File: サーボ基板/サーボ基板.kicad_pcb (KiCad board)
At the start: 2 copper layers, 120 x 170.1 mm, 83 parts, among them J1 Conn_01x02, J10 Conn_02x10, J11 Conn_01x03_Pin, J12 Conn_01x03_Pin, J13 Conn_01x03_Pin, J14 Conn_01x03_Pin, J15 Conn_01x03_Pin, J16 Conn_01x03_Pin, J17 Conn_01x05, J18 Conn_01x05, J19 Conn_01x04, J2 Conn_01x03, J20 Conn_01x04, J21 Conn_01x04, J3 Conn_01x03, J4 Conn_01x03, J5 Conn_01x03, J6 Conn_01x05_Pin, J9 Conn_01x03, SW1 SW_Push, SW2 SW_Push, SW3 SW_Push, SW4 SW_Push, U1 SeeeduinoXIAO RP2040, U10 SN74HC241DW, U2 DEV-16771, U3 SeeeduinoXIAO RP2040, U4 AD8226ARZ, U5 AD8226ARZ, U8 ADuM121N, U9 ADuM121N

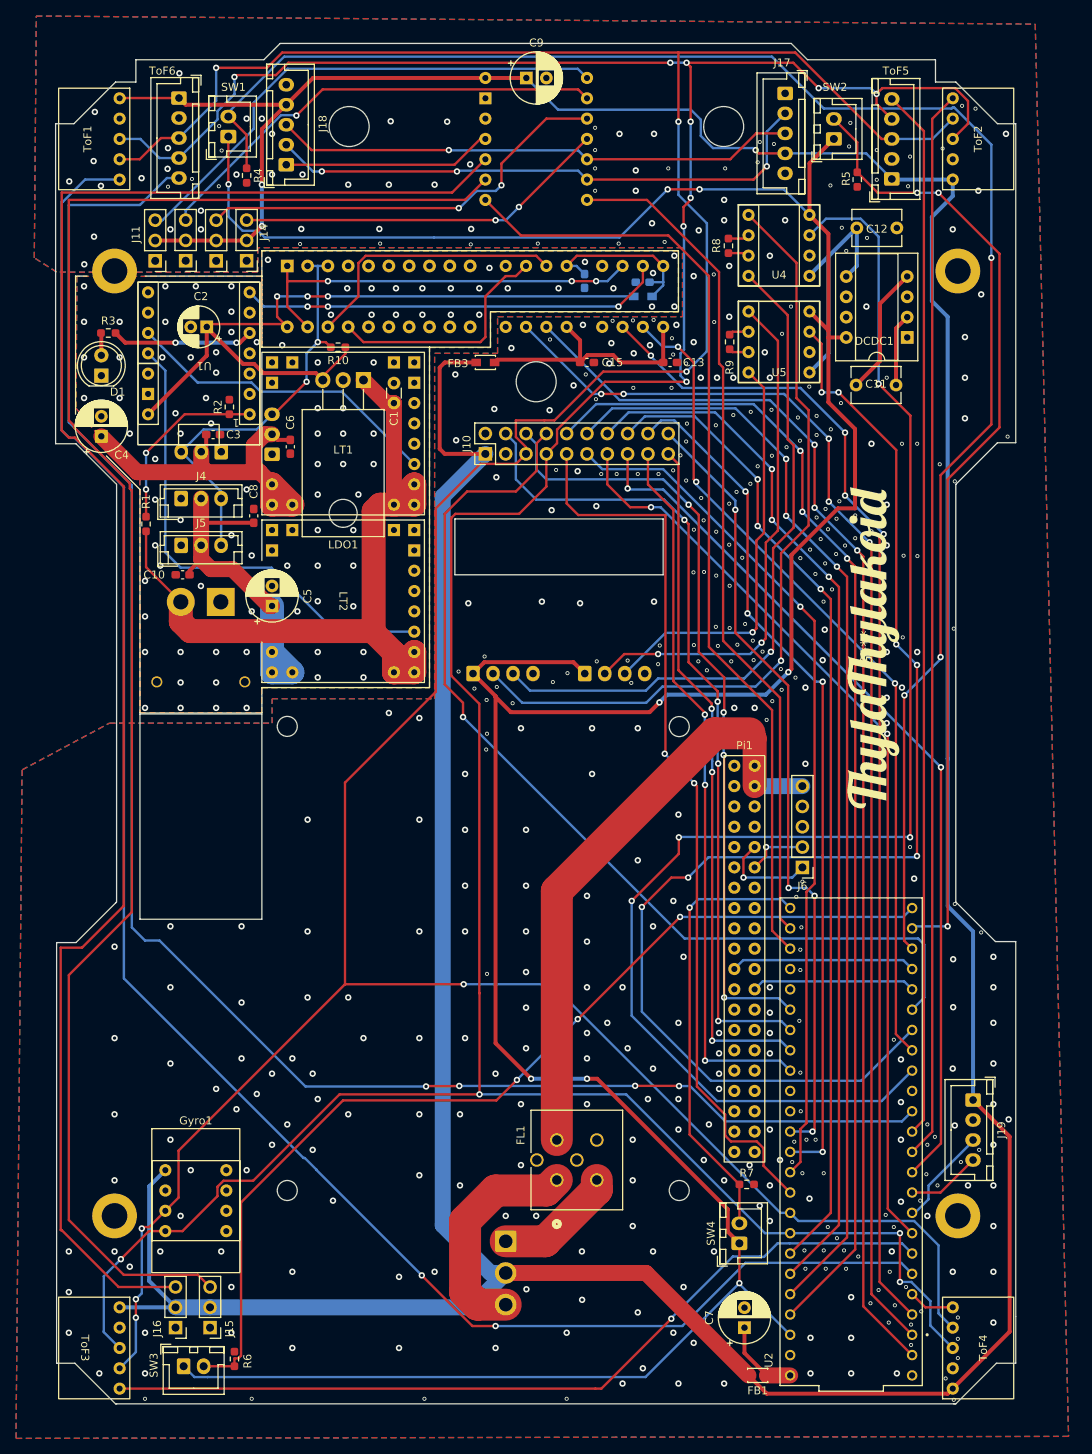
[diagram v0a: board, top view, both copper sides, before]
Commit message: main
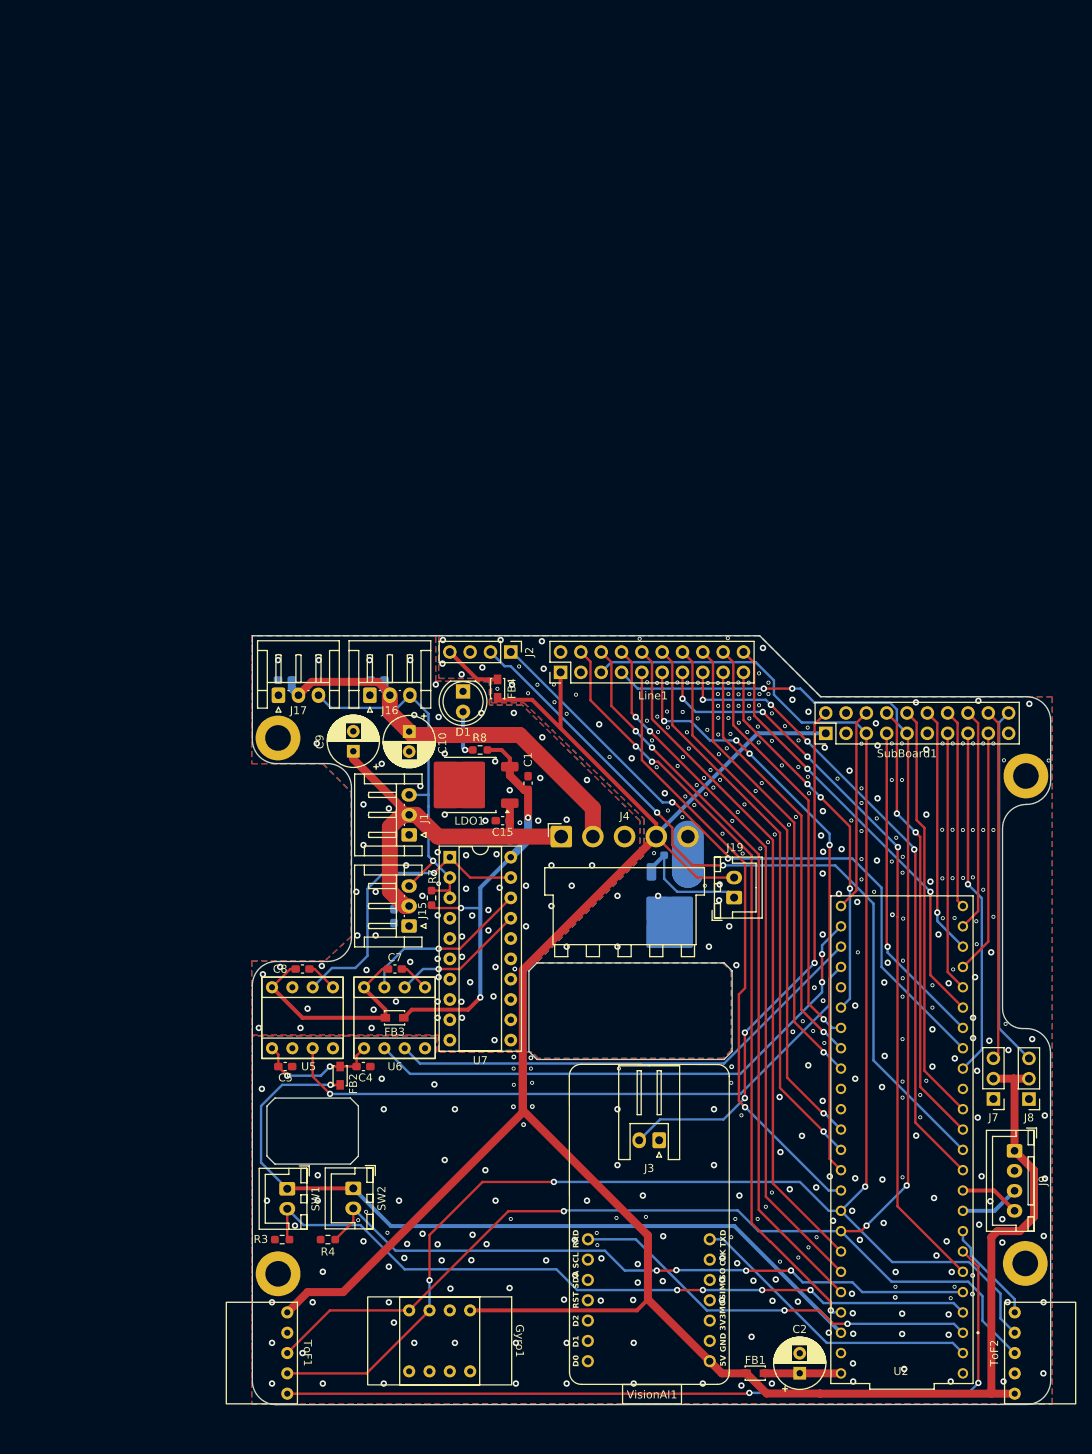
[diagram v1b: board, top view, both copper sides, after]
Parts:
- removed ? (x3): , 
- removed C16: 0.01u, Capacitor_SMD:C_0603_1608Metric_Pad1.08x0.95mm_HandSolder
- removed C3, C6: 0.1u, Capacitor_SMD:C_0603_1608Metric_Pad1.08x0.95mm_HandSolder
- removed DCDC1: ~, Package_DIP:CERDIP-8_W7.62mm_SideBrazed_Socket
- removed FL1: BNX012-01, BNX012-01:BNX012H01_MUR
- removed G***: LOGO, logo:logo
- removed J10: Conn_02x10, Connector_PinHeader_2.54mm:PinHeader_2x10_P2.54mm_Vertical
- removed J11, J12, J13, J14: Conn_01x03_Pin, Connector_PinHeader_2.54mm:PinHeader_1x03_P2.54mm_Vertical
- removed J18: Conn_01x05, Connector_JST:JST_XH_B5B-XH-A_1x05_P2.50mm_Vertical
- removed J20, J21: Conn_01x04, Connector_JST:JST_XH_S4B-XH-A_1x04_P2.50mm_Horizontal
- removed J5: Conn_01x03, Connector_JST:JST_EH_B3B-EH-A_1x03_P2.50mm_Vertical
- removed J6: Conn_01x05_Pin, Connector_PinHeader_2.54mm:PinHeader_1x05_P2.54mm_Vertical
- removed LT1, LT2: ~, LT8640:LT8640
- removed Pi1: RASPBERRY_PI_4B_4GB, Raspberry Pi 5:Raspberry Pi 5
- removed R1: 470, Resistor_SMD:R_0603_1608Metric_Pad0.98x0.95mm_HandSolder
- removed R10, R5, R6: 10k, Resistor_SMD:R_0603_1608Metric_Pad0.98x0.95mm_HandSolder
- removed R2: 220, Resistor_SMD:R_0603_1608Metric_Pad0.98x0.95mm_HandSolder
- removed the REF** at (136.5, 165.1)
- removed the REF** at (101.7, 103.9)
- removed the REF** at (136.5, 47.0)
- removed the REF** at (31.1, 165.1)
- removed the REF** at (31.1, 47.0)
- removed SW3, SW4: SW_Push, Connector_JST:JST_XH_B2B-XH-A_1x02_P2.50mm_Vertical
- removed ToF3, ToF4: ~, ToF:GY530
- removed ToF5, ToF6: ~, Connector_JST:JST_XH_B5B-XH-A_1x05_P2.50mm_Vertical
- removed U1, U3: SeeeduinoXIAO RP2040, XIAO RP2040:XIAO RP2040
- removed U10: SN74HC241DW, Package_DIP:CERDIP-20_W7.62mm_SideBrazed_Socket
- removed U4: AD8226ARZ, MyLibrary:SOP-8_DIP
- removed U8, U9: ADuM121N, MyLibrary:SOP-8_DIP
- added FB4: 100R, Inductor_SMD:L_Walsin_WLFM201209x, F.Cu at (79.0, 99.2)
- added J7: Conn_01x03_Pin, Connector_PinHeader_2.54mm:PinHeader_1x03_P2.54mm_Vertical, F.Cu at (141.0, 150.5)
- added J8: Conn_01x03_Pin, Connector_PinHeader_2.54mm:PinHeader_1x03_P2.54mm_Vertical, F.Cu at (145.4, 150.5)
- added Line1: Conn_02x10, Connector_PinHeader_2.54mm:PinHeader_2x10_P2.54mm_Vertical, F.Cu at (86.9, 97.2)
- added Q1: Q_NMOS_GDS, Package_TO_SOT_SMD:TO-252-2, B.Cu at (100.5, 127.1)
- added REF**: MountingHole_3.2mm_M3_DIN965_Pad, MountingHole:MountingHole_3.2mm_M3_DIN965_Pad, F.Cu at (51.5, 105.4)
- added REF**: MountingHole_3.2mm_M3_DIN965_Pad, MountingHole:MountingHole_3.2mm_M3_DIN965_Pad, F.Cu at (51.6, 172.3)
- added REF**: MountingHole_3.2mm_M3_DIN965_Pad, MountingHole:MountingHole_3.2mm_M3_DIN965_Pad, F.Cu at (145.0, 110.1)
- added REF**: MountingHole_3.2mm_M3_DIN965_Pad, MountingHole:MountingHole_3.2mm_M3_DIN965_Pad, F.Cu at (145.0, 171.0)
- added SubBoard1: Conn_02x10, Connector_PinHeader_2.54mm:PinHeader_2x10_P2.54mm_Vertical, F.Cu at (120.0, 104.8)
- added U6: ADuM121N, MyLibrary:SOP-8_DIP, F.Cu at (66.1, 140.3)
- added U7: SN74HC241DW, Package_DIP:CERDIP-20_W7.62mm_SideBrazed_Socket, F.Cu at (73.0, 120.3)
- added VisionAI1: ~, MyLibrary:Grove Vision AI V2, F.Cu at (98.3, 175.9)
- C1: value 0.33uF -> 2.2u; footprint Capacitor_THT:C_Disc_D3.0mm_W1.6mm_P2.50mm -> Capacitor_SMD:C_0603_1608Metric_Pad1.08x0.95mm_HandSolder
- C10: value 0.1u -> 100u; footprint Capacitor_SMD:C_0603_1608Metric_Pad1.08x0.95mm_HandSolder -> Capacitor_THT:CP_Radial_D6.3mm_P2.50mm
- C11, C12: value 10u -> 0.1u; footprint Capacitor_THT:C_Disc_D6.0mm_W4.4mm_P5.00mm -> Capacitor_SMD:C_0603_1608Metric_Pad1.08x0.95mm_HandSolder; moved to B.Cu
- C13: value 0.01u -> 0.1u; moved to B.Cu
- C14: value 0.01u -> 0.1u
- C15: value 0.01u -> 0.33uF
- C2: value 33uF -> 100u; footprint Capacitor_THT:CP_Radial_D5.0mm_P2.00mm -> Capacitor_THT:CP_Radial_D6.3mm_P2.50mm
- C4, C5, C7: value 100u -> 0.01u; footprint Capacitor_THT:CP_Radial_D6.3mm_P2.50mm -> Capacitor_SMD:C_0603_1608Metric_Pad1.08x0.95mm_HandSolder
- C8: value 0.1u -> 0.01u
- FB2: moved to F.Cu
- J1: value Conn_01x02 -> Conn_01x03; footprint Connector_AMASS:AMASS_XT30PW-M_1x02_P2.50mm_Horizontal -> Connector_JST:JST_EH_S3B-EH_1x03_P2.50mm_Horizontal; moved to F.Cu
- J15, J16: value Conn_01x03_Pin -> Conn_01x03; footprint Connector_PinHeader_2.54mm:PinHeader_1x03_P2.54mm_Vertical -> Connector_JST:JST_EH_S3B-EH_1x03_P2.50mm_Horizontal
- J17: value Conn_01x05 -> Conn_01x03; footprint Connector_JST:JST_XH_B5B-XH-A_1x05_P2.50mm_Vertical -> Connector_JST:JST_EH_S3B-EH_1x03_P2.50mm_Horizontal
- J19: value Conn_01x04 -> Power Switch; footprint Connector_JST:JST_XH_B4B-XH-A_1x04_P2.50mm_Vertical -> Connector_JST:JST_XH_B2B-XH-A_1x02_P2.50mm_Vertical
- J2: value Conn_01x03 -> Conn_01x04_Pin; footprint Connector_JST:JST_EH_S3B-EH_1x03_P2.50mm_Horizontal -> Connector_PinHeader_2.54mm:PinHeader_1x04_P2.54mm_Vertical; moved to F.Cu
- J3: value Conn_01x03 -> Conn_01x02_Pin; footprint Connector_JST:JST_EH_S3B-EH_1x03_P2.50mm_Horizontal -> Connector_JST:JST_XH_S2B-XH-A_1x02_P2.50mm_Horizontal; moved to F.Cu
- J4: value Conn_01x03 -> PWR OUT; footprint Connector_JST:JST_EH_B3B-EH-A_1x03_P2.50mm_Vertical -> Connector_JST:JST_VH_B5PS-VH_1x05_P3.96mm_Horizontal
- J9: value Conn_01x03 -> Conn_01x04; footprint Connector_JST:JST_VH_B3PS-VH_1x03_P3.96mm_Horizontal -> Connector_JST:JST_XH_B4B-XH-A_1x04_P2.50mm_Vertical; moved to F.Cu
- LDO1: footprint Package_TO_SOT_THT:TO-220-3_Horizontal_TabDown -> Package_TO_SOT_SMD:TO-252-2
- R3: value 220 -> 10k
- R8: value 50 -> 220
- R9: value 50 -> 1k; moved to B.Cu
- U5: value AD8226ARZ -> ADuM121N
- moved ToF1 153.2 mm to (52.7, 182.2)
- moved ToF2 152.0 mm to (143.6, 182.2)
- moved C2 150.3 mm to (116.8, 184.8), turned to 90 degrees
- moved SW2 144.3 mm to (61.0, 161.7), turned to -90 degrees
- moved R4 133.4 mm to (57.8, 168.1), turned to 180 degrees
- moved SW1 131.7 mm to (52.7, 161.7), turned to -90 degrees
- moved R3 115.4 mm to (52.1, 168.1)
- moved C12 106.5 mm to (66.0, 127.6), turned to 90 degrees
- moved FB2 104.5 mm to (59.3, 147.6), turned to -90 degrees
- moved U5 103.4 mm to (54.6, 140.3), turned to 90 degrees
- moved J3 102.0 mm to (99.2, 155.6)
- moved J17 98.3 mm to (51.6, 100.0), turned to 0 degrees
- moved C9 86.9 mm to (61.0, 107.0), turned to 90 degrees
- moved C4 85.3 mm to (62.2, 146.4), turned to 0 degrees
- moved C11 83.6 mm to (66.0, 116.5), turned to 90 degrees
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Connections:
- net /main/scl renamed /scl
- net /main/sda renamed /sda
- C1 pad 1: VDD -> GND
- C1 pad 2: GND -> +5V
- C10 pad 1: GND -> /6VB
- C10 pad 2: Net-(J4-Pin_2) -> GND
- C11 pad 1: Net-(DCDC1-CAP+) -> GND
- C11 pad 2: Net-(DCDC1-CAP-) -> /6VA
- C12 pad 1: GND2 -> GND
- C12 pad 2: VEE -> /6VA
- C13 pad 1: Net-(U8-VDD1) -> GND
- C13 pad 2: GND2 -> /6VB
- C14 pad 1: Net-(U8-VDD2) -> GND
- C14 pad 2: GND -> /6VB
- C15 pad 1: Net-(U8-VDD1) -> /6VA
- C15 pad 2: GND2 -> GND
- C2 pad 1: +5V -> Net-(C2-Pad1)
- C2 pad 2: GND -> GND2
- C4 pad 1: Net-(J2-Pin_2) -> Net-(U5-VDD1)
- C4 pad 2: GND -> GND2
- C5 pad 1: Net-(J4-Pin_2) -> Net-(U5-VDD1)
- C5 pad 2: GND -> GND2
- C7 pad 1: Net-(C7-Pad1) -> Net-(U5-VDD2)
- C7 pad 2: GND2 -> GND
- C8 pad 2: Net-(J4-Pin_2) -> Net-(U5-VDD2)
- C9 pad 1: +5VA -> /6VA
- C9 pad 2: GND2 -> GND
- FB1 pad 2: Net-(C7-Pad1) -> Net-(C2-Pad1)
- FB2 pad 1: +5V -> Net-(U5-VDD1)
- FB2 pad 2: Net-(U8-VDD2) -> +3.3V
- FB3 pad 1: Net-(U8-VDD1) -> +5V
- FB3 pad 2: +5VA -> Net-(U5-VDD2)
- J1 pad 2: VDD -> /6VA
- J15 pad 1: GND2 -> GND
- J15 pad 2: +5VA -> /6VA
- J15 pad 3: /main/PWM5 -> DATA
- J16 pad 1: GND2 -> GND
- J16 pad 2: +5VA -> /6VB
- J16 pad 3: /main/PWM6 -> DATA
- J17 pad 1: unconnected-(J17-Pin_1-Pad1) -> GND
- J17 pad 2: /main/scl_sub -> /6VB
- J17 pad 3: /main/sda_sub -> DATA
- J19 pad 1: +5VA -> Net-(J19-Pin_1)
- J19 pad 2: GND2 -> +5VA
- J2 pad 1: GND -> /LiDAR_TX
- J2 pad 2: Net-(J2-Pin_2) -> /LiDAR_PWM
- J2 pad 3: DATA -> GND2
- J3 pad 1: GND -> GND2
- J3 pad 2: Net-(J2-Pin_2) -> /tx
- J4 pad 1: GND -> /6VA
- J4 pad 2: Net-(J4-Pin_2) -> /6VB
- J4 pad 3: DATA -> GND
- J9 pad 1: Net-(J9-Pin_1) -> +5VA
- J9 pad 2: +5VA -> GND2
- J9 pad 3: Net-(J9-Pin_3) -> /rx2_main
- LDO1 pad 1: VDD -> /6VA
- R3 pad 1: /RED LED -> /LimSW1
- R3 pad 2: Net-(D1-A) -> GND2
- R4 pad 1: /main/LimSW1 -> /LimSW2
- R7 pad 1: /main/LimSW4 -> DATA
- R7 pad 2: GND2 -> +5V
- R8 pad 1: Net-(R8-Pad1) -> +5V
- R8 pad 2: Net-(R8-Pad2) -> Net-(D1-A)
- R9 pad 1: Net-(R9-Pad1) -> Net-(J19-Pin_1)
- R9 pad 2: Net-(R9-Pad2) -> Net-(J4-Pin_5)
- SW1 pad 2: /main/LimSW1 -> /LimSW1
- SW2 pad 2: /main/LimSW2 -> /LimSW2
- ToF1 pad 5: /main/xshut3 -> /xshut3
- ToF2 pad 5: /main/xshut5 -> /xshut4
- U2 pad 0: /main/rx_dxl -> /rx7_main
- U2 pad 1: /main/tx_dxl -> /tx7_main
- U2 pad 10: /main/xshut5 -> /LiDAR_PWM
- U2 pad 11: /main/xshut7 -> /xshut7
- U2 pad 12: /main/xshut8 -> /xshut6
- U2 pad 14: /main/Line3 -> /Line6
- U2 pad 15: /main/Line4 -> /Line7
- U2 pad 16: /main/scl1 -> /scl1
- U2 pad 17: /main/sda1 -> /sda1
- U2 pad 2: /main/tx_en -> /LimSW1
- U2 pad 20: /main/Line5 -> /Line8
- U2 pad 21: /main/Line6 -> /Line9
- U2 pad 22: /main/Line7 -> /Line10
- U2 pad 23: /main/Line8 -> /Line11
- U2 pad 24: /main/loadcell1 -> /loadcell1
- U2 pad 25: /main/rx_main_power -> /LiDAR_TX
- U2 pad 26: /main/loadcell2 -> /loadcell2
- U2 pad 27: /main/Line9 -> /Line3
- U2 pad 28: /main/rx7_main -> /rx8_main
- U2 pad 29: /main/rx3_pi5 -> /tx8_main
- U2 pad 3: /main/xshut6 -> /LimSW2
- U2 pad 30: /main/LimSW1 -> /xshut5
- U2 pad 31: /main/LimSW2 -> /LimSW4
- U2 pad 32: /main/LimSW3 -> /LimSW3
- U2 pad 33: /main/LimSW4 -> /xshut8
- U2 pad 34: /main/rx8_main -> /rx_dxl
- U2 pad 35: /main/rx_sub -> /tx_dxl
- U2 pad 36: unconnected-(U2-CS2-Pad36) -> /tx_en
- U2 pad 38: /main/Line10 -> /Line2
- U2 pad 39: /main/Line11 -> /Line4
- U2 pad 4: /main/xshut3 -> /xshut1
- U2 pad 40: /main/Line2 -> /Line1
- U2 pad 41: /main/Line1 -> /Line5
- U2 pad 5: /main/xshut4 -> /xshut3
- U2 pad 6: /main/xshut1 -> /xshut4
- U2 pad 7: /main/rx2_main -> /rx2_main
- U2 pad 8: /main/tx2_main -> /tx2_main
- U2 pad 9: /main/xshut2 -> /xshut2
- U2 pad VIN: Net-(C7-Pad1) -> Net-(C2-Pad1)
- U5 pad 1: /main/LdCl_WHITE2 -> Net-(U5-VDD1)
- U5 pad 2: Net-(R9-Pad1) -> unconnected-(U5-VOA-Pad2)
- U5 pad 3: Net-(R9-Pad2) -> /tx_en
- U5 pad 4: /main/LdCl_GREEN2 -> GND2
- U5 pad 5: VEE -> GND
- U5 pad 6: GND2 -> Net-(U5-VOB)
- U5 pad 7: /main/loadcell2 -> unconnected-(U5-VIA-Pad7)
- U5 pad 8: +3.3V -> Net-(U5-VDD2)
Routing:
- net +3.3V: track 401.6 -> 99.3 mm, vias 8 -> 1
- net +5VA: track 563.8 -> 312.7 mm, vias 3 -> 0
- net /main/xshut3: track 229.5 -> 0.00 mm, vias 2 -> 0
- net /main/xshut8: track 216.9 -> 0.00 mm, vias 4 -> 0
- net /main/LimSW1: track 216.3 -> 0.00 mm, vias 3 -> 0
- net /sda: track 426.0 -> 215.4 mm, vias 7 -> 3
- net /scl: track 425.1 -> 214.6 mm, vias 13 -> 5
- net /main/PWM6: track 210.2 -> 0.00 mm
- net /main/PWM5: track 208.3 -> 0.00 mm
- net /main/loadcell1: track 181.9 -> 0.00 mm, vias 4 -> 0
- net /main/loadcell2: track 162.4 -> 0.00 mm, vias 7 -> 0
- net /main/tx_dxl: track 160.0 -> 0.00 mm, vias 5 -> 0
- net /main/rx_dxl: track 158.5 -> 0.00 mm, vias 3 -> 0
- net /main/tx_en: track 147.5 -> 0.00 mm, vias 4 -> 0
- net /main/Line8: track 147.3 -> 0.00 mm, vias 3 -> 0
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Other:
- board size 120 x 170.1 mm -> 99.8 x 96.1 mm
